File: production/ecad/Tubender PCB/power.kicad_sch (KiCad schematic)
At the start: 46 parts, among them Q1 CSD19502Q5B, Q2 CSD19534Q5A, U1 LMR36520FADDAR, U2 LM5146RGYR, U3 MCP23017-E_SO

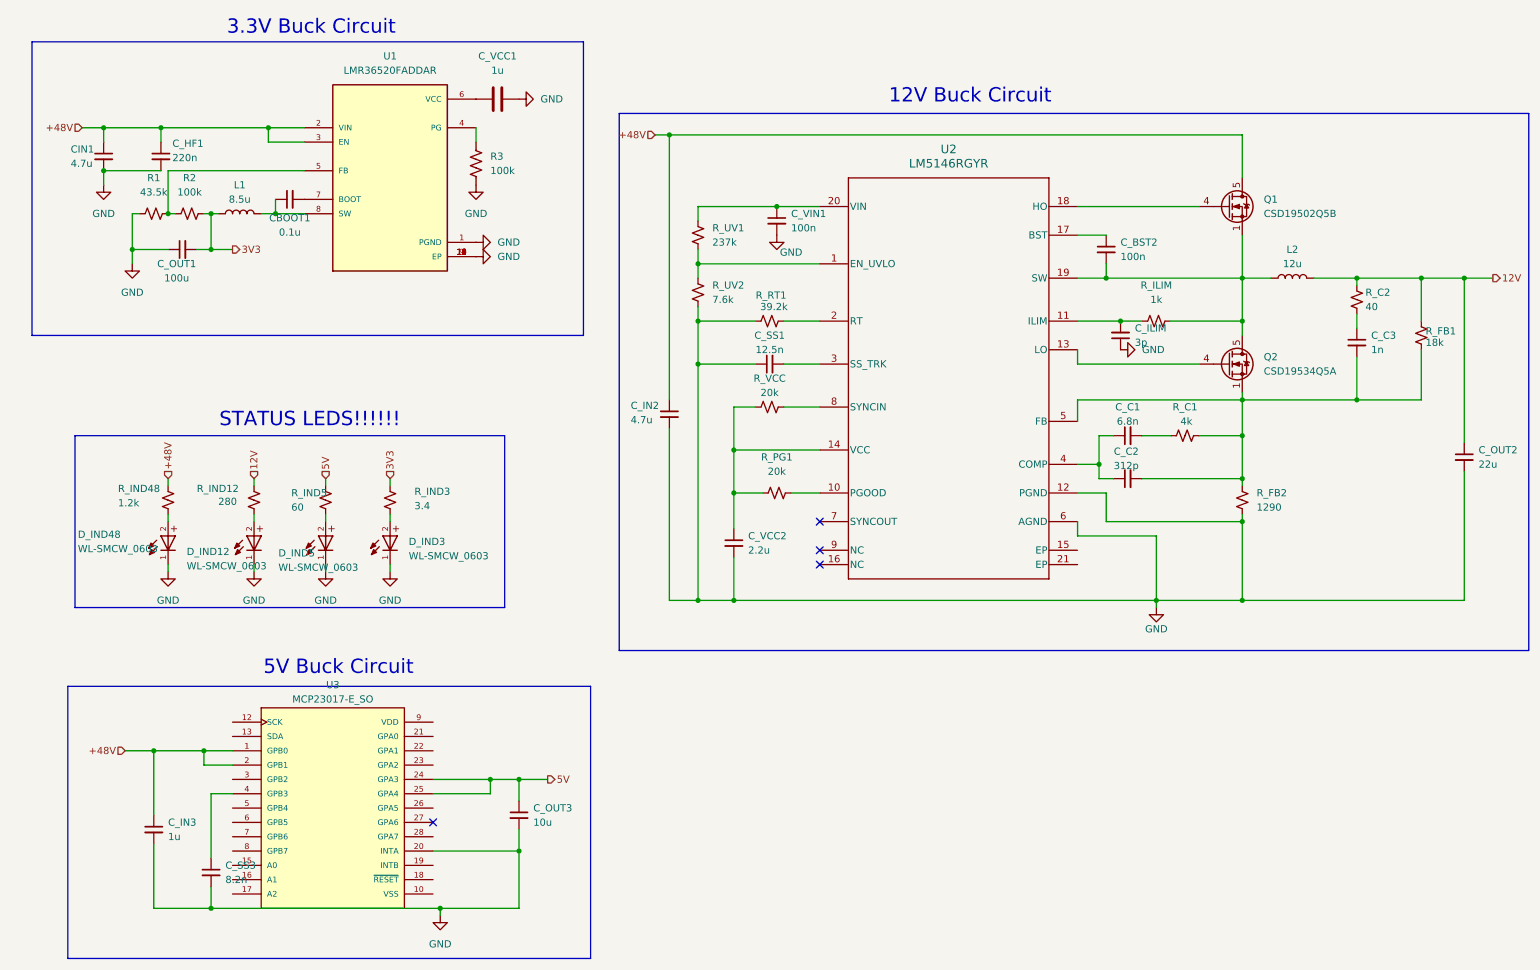
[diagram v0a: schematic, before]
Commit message: Formatting
Boom
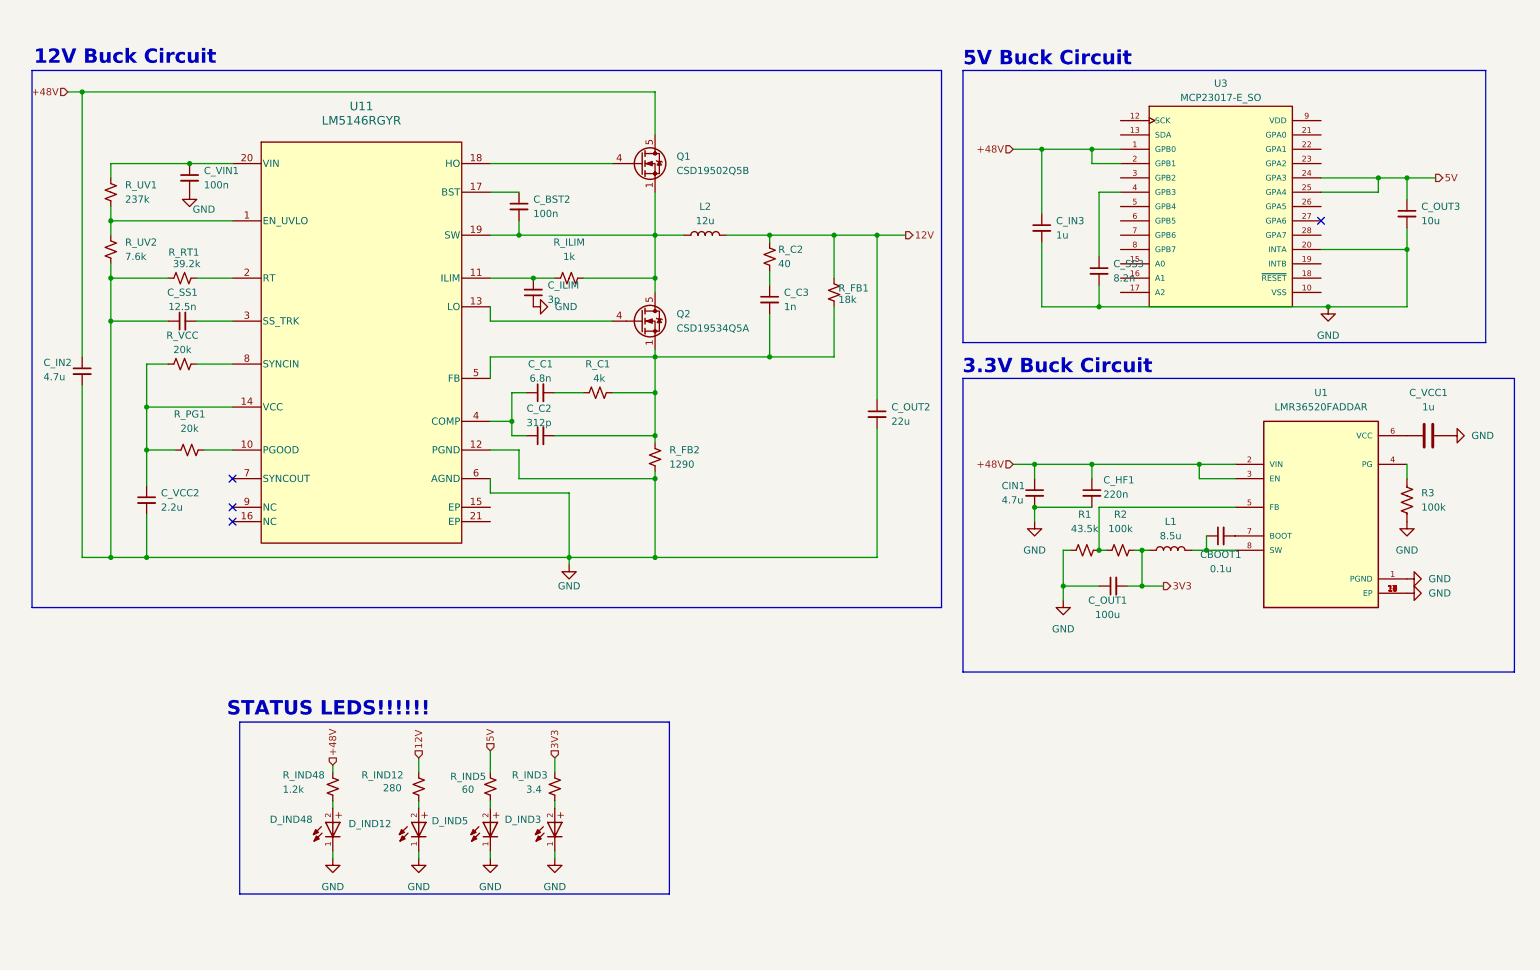
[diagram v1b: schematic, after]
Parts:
- renumbered U2 to U11
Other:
- moved on the sheet: CBOOT1, CIN1, C_BST2, C_C1, C_C2, C_C3, C_HF1, C_ILIM, C_IN2, C_IN3, C_OUT1, C_OUT2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
